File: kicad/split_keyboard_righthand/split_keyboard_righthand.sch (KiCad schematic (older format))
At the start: 94 parts, among them J1 Conn_02x08_Odd_Even, SW1 SW_PUSH, SW10 SW_PUSH, SW11 SW_PUSH, SW12 SW_PUSH, SW13 SW_PUSH, SW14 SW_PUSH, SW15 SW_PUSH, SW16 SW_PUSH, SW17 SW_PUSH, SW18 SW_PUSH, SW19 SW_PUSH, SW2 SW_PUSH, SW20 SW_PUSH, SW21 SW_PUSH, SW22 SW_PUSH, SW23 SW_PUSH, SW24 SW_PUSH, SW25 SW_PUSH, SW26 SW_PUSH, SW27 SW_PUSH, SW28 SW_PUSH, SW29 SW_PUSH, SW3 SW_PUSH, SW30 SW_PUSH, SW31 SW_PUSH, SW32 SW_PUSH, SW33 SW_PUSH, SW34 SW_PUSH, SW35 SW_PUSH, SW36 SW_PUSH, SW37 SW_PUSH, SW38 SW_PUSH, SW39 SW_PUSH, SW4 SW_PUSH, SW40 SW_PUSH, SW41 SW_PUSH, SW42 SW_PUSH, SW43 SW_PUSH, SW44 SW_PUSH, SW45 SW_PUSH, SW5 SW_PUSH, SW6 SW_PUSH, SW7 SW_PUSH, SW8 SW_PUSH, SW9 SW_PUSH

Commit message: complete lefthand pcb.
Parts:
- D46: footprint LED_THT:LED_D1.8mm_W1.8mm_H2.4mm_Horizontal_O3.81mm_Z1.6mm -> LED_THT:LED_D3.0mm_FlatTop
- R1: footprint kbd:R -> Resistor_THT:R_Axial_DIN0207_L6.3mm_D2.5mm_P7.62mm_Horizontal
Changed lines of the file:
@@
 F 0 "D46" H 3143 6145 50  0000 C CNN
 F 1 "LED" H 3143 6236 50  0000 C CNN
-F 2 "LED_THT:LED_D1.8mm_W1.8mm_H2.4mm_Horizontal_O3.81mm_Z1.6mm" H 3150 6400 50  0001 C CNN
+F 2 "LED_THT:LED_D3.0mm_FlatTop" H 3150 6400 50  0001 C CNN
 F 3 "~" H 3150 6400 50  0001 C CNN
 	1    3150 6400
@@
 F 0 "R1" V 3243 6400 50  0000 C CNN
 F 1 "R" V 3334 6400 50  0000 C CNN
-F 2 "kbd:R" V 3380 6400 50  0001 C CNN
+F 2 "Resistor_THT:R_Axial_DIN0207_L6.3mm_D2.5mm_P7.62mm_Horizontal" V 3380 6400 50  0001 C CNN
 F 3 "~" H 3450 6400 50  0001 C CNN
 	1    3450 6400

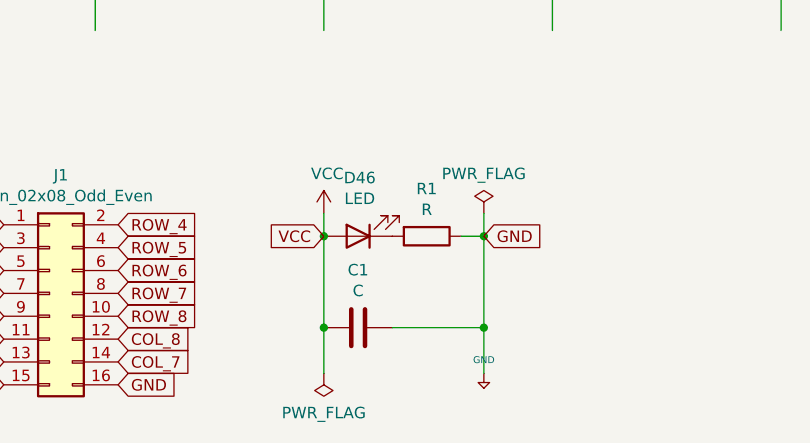
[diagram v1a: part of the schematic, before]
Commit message: complete to design pcb, and export gerber data.
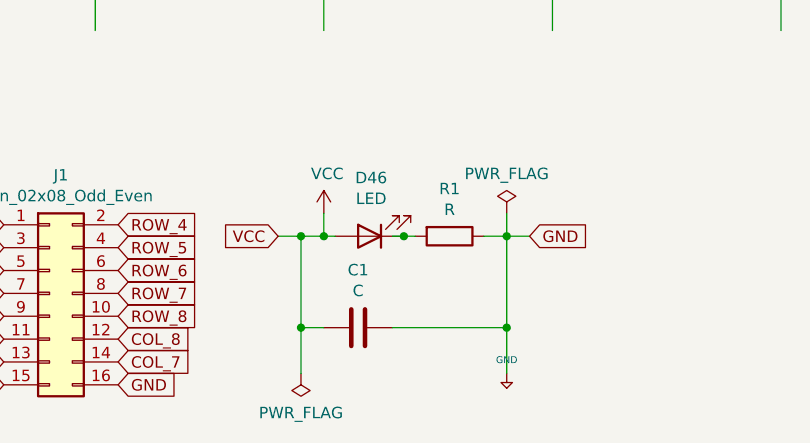
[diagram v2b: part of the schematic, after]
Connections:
- wire segments 107 -> 114
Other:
- moved on the sheet: D46, R1
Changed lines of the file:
@@
 L keyboard_parts:GND #PWR0102
 U 1 1 5FBB32F2
-P 3700 7000
-F 0 "#PWR0102" H 3700 7050 20  0001 C CNN
-F 1 "GND" H 3700 7059 30  0000 C CNN
-F 2 "" H 3700 7000 60  0000 C CNN
-F 3 "" H 3700 7000 60  0000 C CNN
-	1    3700 7000
+P 3800 7000
+F 0 "#PWR0102" H 3800 7050 20  0001 C CNN
+F 1 "GND" H 3800 7059 30  0000 C CNN
+F 2 "" H 3800 7000 60  0000 C CNN
+F 3 "" H 3800 7000 60  0000 C CNN
+	1    3800 7000
 	1    0    0    -1
 $EndComp
@@
 L power:PWR_FLAG #FLG0101
 U 1 1 5FBBADC9
-P 3700 6300
-F 0 "#FLG0101" H 3700 6375 50  0001 C CNN
-F 1 "PWR_FLAG" H 3700 6473 50  0000 C CNN
-F 2 "" H 3700 6300 50  0001 C CNN
-F 3 "~" H 3700 6300 50  0001 C CNN
-	1    3700 6300
+P 3800 6300
+F 0 "#FLG0101" H 3800 6375 50  0001 C CNN
+F 1 "PWR_FLAG" H 3800 6473 50  0000 C CNN
+F 2 "" H 3800 6300 50  0001 C CNN
+F 3 "~" H 3800 6300 50  0001 C CNN
+	1    3800 6300
 	1    0    0    -1
 $EndComp
@@
 L power:PWR_FLAG #FLG0102
 U 1 1 5FBBBFBC
-P 3000 7000
-F 0 "#FLG0102" H 3000 7075 50  0001 C CNN
-F 1 "PWR_FLAG" H 3000 7173 50  0000 C CNN
-F 2 "" H 3000 7000 50  0001 C CNN
-F 3 "~" H 3000 7000 50  0001 C CNN
-	1    3000 7000
+P 2900 7000
+F 0 "#FLG0102" H 2900 7075 50  0001 C CNN
+F 1 "PWR_FLAG" H 2900 7173 50  0000 C CNN
+F 2 "" H 2900 7000 50  0001 C CNN
+F 3 "~" H 2900 7000 50  0001 C CNN
+	1    2900 7000
 	-1   0    0    1
 $EndComp
@@
 L Device:LED D46
 U 1 1 5FBC96F2
-P 3150 6400
-F 0 "D46" H 3143 6145 50  0000 C CNN
-F 1 "LED" H 3143 6236 50  0000 C CNN
-F 2 "LED_THT:LED_D3.0mm_FlatTop" H 3150 6400 50  0001 C CNN
-F 3 "~" H 3150 6400 50  0001 C CNN
-	1    3150 6400
+P 3200 6400
+F 0 "D46" H 3193 6145 50  0000 C CNN
+F 1 "LED" H 3193 6236 50  0000 C CNN
+F 2 "LED_THT:LED_D3.0mm_FlatTop" H 3200 6400 50  0001 C CNN
+F 3 "~" H 3200 6400 50  0001 C CNN
+	1    3200 6400
 	-1   0    0    1
 $EndComp
 Wire Wire Line
 	3000 6300 3000 6400
-Connection ~ 3000 6400
 $Comp
 L Device:R R1
 U 1 1 5FBD025D
-P 3450 6400
-F 0 "R1" V 3243 6400 50  0000 C CNN
-F 1 "R" V 3334 6400 50  0000 C CNN
-F 2 "Resistor_THT:R_Axial_DIN0207_L6.3mm_D2.5mm_P7.62mm_Horizontal" V 3380 6400 50  0001 C CNN
-F 3 "~" H 3450 6400 50  0001 C CNN
-	1    3450 6400
+P 3550 6400
+F 0 "R1" V 3343 6400 50  0000 C CNN
+F 1 "R" V 3434 6400 50  0000 C CNN
+F 2 "Resistor_THT:R_Axial_DIN0207_L6.3mm_D2.5mm_P7.62mm_Horizontal" V 3480 6400 50  0001 C CNN
+F 3 "~" H 3550 6400 50  0001 C CNN
+	1    3550 6400
 	0    1    1    0
 $EndComp
@@
 $EndComp
 Wire Wire Line
-	3000 6400 3000 6800
-Connection ~ 3000 6800
+	3800 6300 3800 6400
+Connection ~ 3800 6800
 Wire Wire Line
-	3000 6800 3000 7000
+	3800 6800 3800 7000
 Wire Wire Line
-	3700 6300 3700 6400
+	3700 6400 3800 6400
+Connection ~ 3800 6400
 Wire Wire Line
-	3300 6800 3700 6800
-Connection ~ 3700 6800
-Wire Wire Line
-	3700 6800 3700 7000
-Wire Wire Line
-	3600 6400 3700 6400
-Connection ~ 3700 6400
-Wire Wire Line
-	3700 6400 3700 6800
-Text GLabel 3000 6400 0    50   Input ~ 0
+	3800 6400 3800 6800
+Text GLabel 2800 6400 0    50   Input ~ 0
 VCC
-Text GLabel 3700 6400 2    50   Input ~ 0
+Text GLabel 3900 6400 2    50   Input ~ 0
 GND
 Text GLabel 1500 3700 0    50   Input ~ 0
@@
 Text GLabel 1500 2300 0    50   Input ~ 0
 ROW_4
+Wire Wire Line
+	2900 6400 2900 6800
+Wire Wire Line
+	2900 6400 3000 6400
+Connection ~ 3000 6400
+Wire Wire Line
+	3000 6800 2900 6800
+Connection ~ 2900 6800
+Wire Wire Line
+	2900 6800 2900 7000
+Connection ~ 2900 6400
+Wire Wire Line
+	2800 6400 2900 6400
+Wire Wire Line
+	3800 6400 3900 6400
+Wire Wire Line
+	3300 6400 3350 6400
+Wire Wire Line
+	3300 6800 3800 6800
+Connection ~ 3350 6400
+Wire Wire Line
+	3350 6400 3400 6400
+Wire Wire Line
+	3050 6400 3000 6400
 $EndSCHEMATC
